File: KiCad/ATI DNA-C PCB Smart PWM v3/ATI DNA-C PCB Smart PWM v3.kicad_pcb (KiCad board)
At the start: 2 copper layers, 70 x 20 mm, 17 parts, among them U1 SmartPWMv3

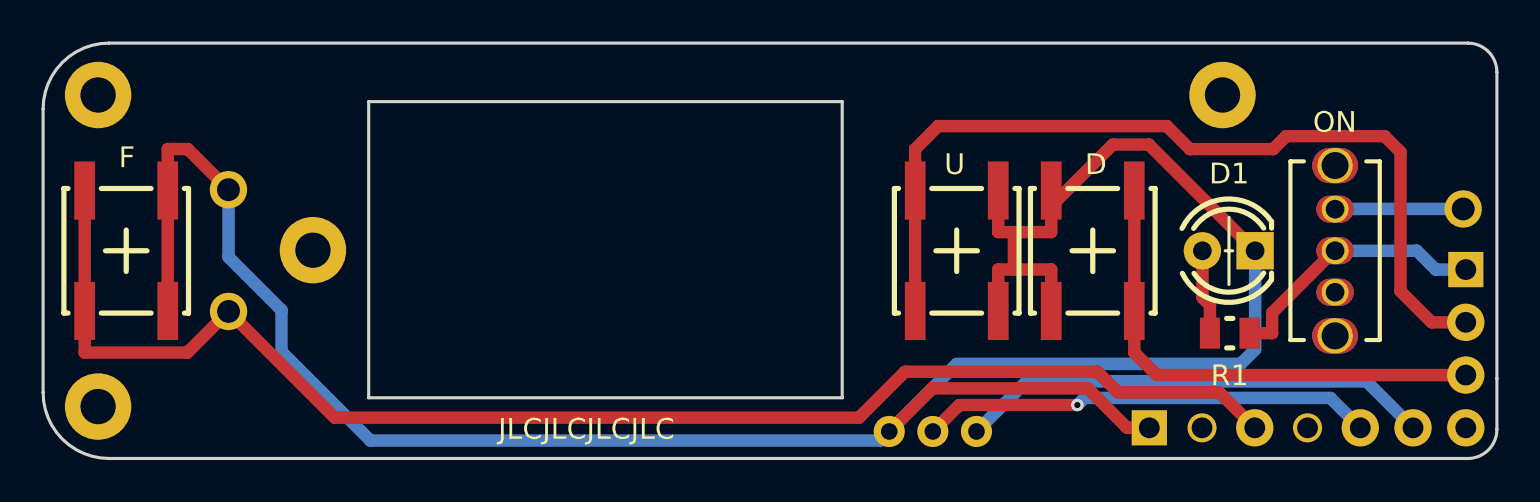
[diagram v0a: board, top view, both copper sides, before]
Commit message: Make pretty
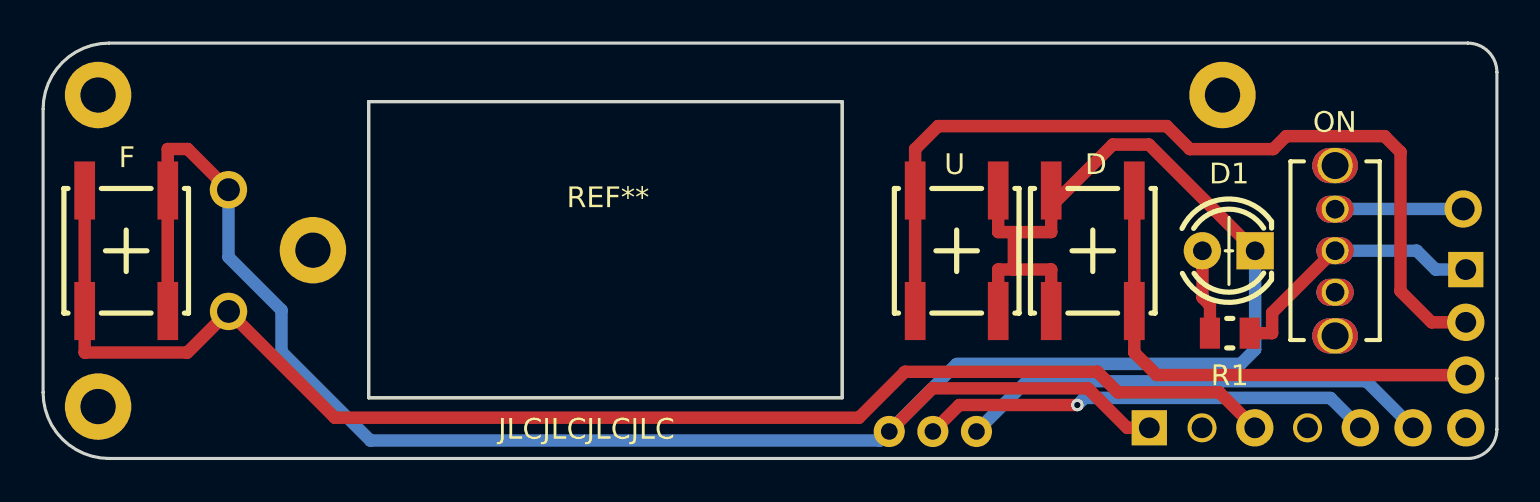
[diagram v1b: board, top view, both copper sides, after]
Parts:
- added REF**: 0.36_inch_VM, ATI DNA-C PCB Smart PWM v3:0.36_inch_VM, F.Cu at (141.7, 100.3)
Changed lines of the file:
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@@
     (tracks 81)
     (zones 0)
-    (modules 17)
+    (modules 18)
     (nets 16)
   )
@@
     (add_net "Net-(U1-Pad9)")
   )
+  (module "ATI DNA-C PCB Smart PWM v3:0.36_inch_VM" (layer F.Cu)
+    (at 141.72 100.27)
+    (fp_text reference REF** (at 0 -2.69) (layer F.SilkS)
+      (effects (font (size 1 1) (thickness 0.15)))
+    )
+    (fp_text value 0.36_inch_VM (at 0 -0.73) (layer F.Fab) hide
+      (effects (font (size 1 1) (thickness 0.15)))
+    )
+    (fp_line (start 11.2781 -7.3084) (end -11.5219 -7.3084) (layer F.SilkS) (width 0.15))
+    (fp_line (start -11.5219 -7.3084) (end -11.5219 6.9516) (layer F.SilkS) (width 0.15))
+    (fp_line (start -11.5219 6.9516) (end 11.2781 6.9516) (layer F.SilkS) (width 0.15))
+    (fp_line (start 11.2781 6.9516) (end 11.2781 -7.3084) (layer F.SilkS) (width 0.15))
+    (model "${KIPRJMOD}/ATI DNA-C PCB Smart PWM v3.pretty/XDxx09x3.step"
+      (offset (xyz -0.1 0.15 4.45))
+      (scale (xyz 1.018 1 1.022))
+      (rotate (xyz -90 0 0))
+    )
+  )
   (module "ATI DNA-C PCB Smart PWM v3:PAD_24G" (layer F.Cu)
